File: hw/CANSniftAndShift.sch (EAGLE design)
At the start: 41 parts, among them CON1 FCI-10033526-N3212LF, CON4 FCI-10033526-N3212LF, IC3 TJA1050, IC4 TJA1050, IC7 FT232RL, Q1 16MHz

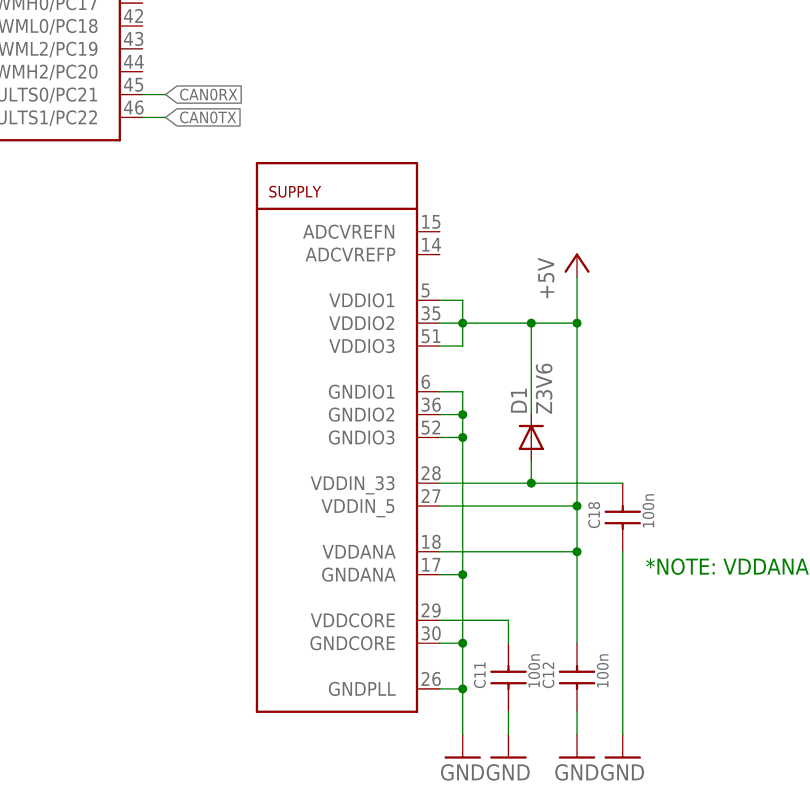
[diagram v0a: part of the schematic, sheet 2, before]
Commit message: sw modified
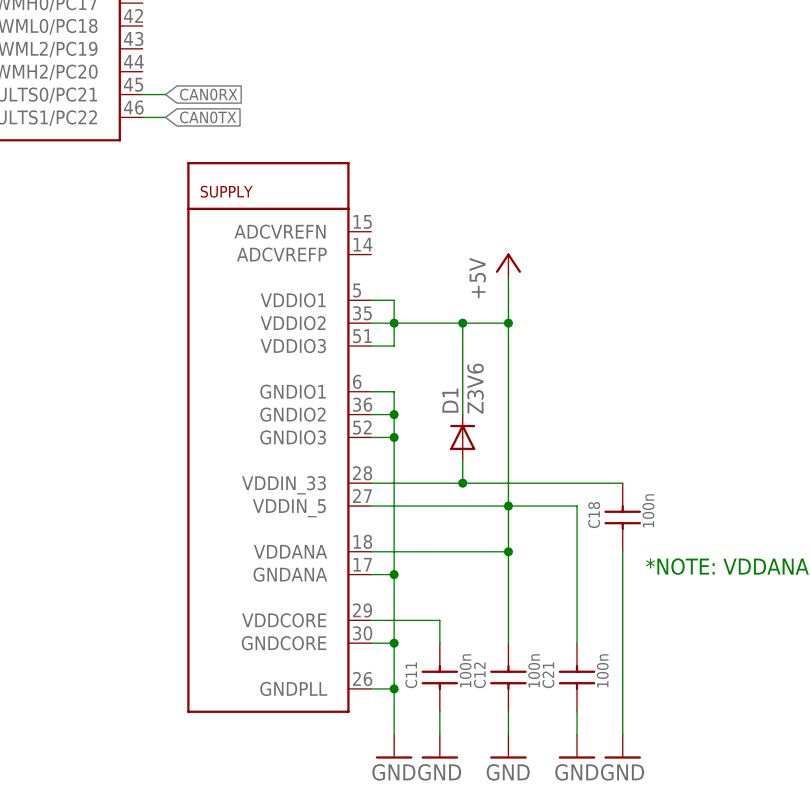
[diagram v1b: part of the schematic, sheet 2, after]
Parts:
- added C21: 100n, SchlegelAr_Master:C_SMD0603
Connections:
- net +5V: now also C21.P$2
- net GND: now also C21.P$1
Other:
- moved on the sheet: C11, C12, D1
